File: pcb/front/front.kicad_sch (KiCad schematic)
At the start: 187 parts

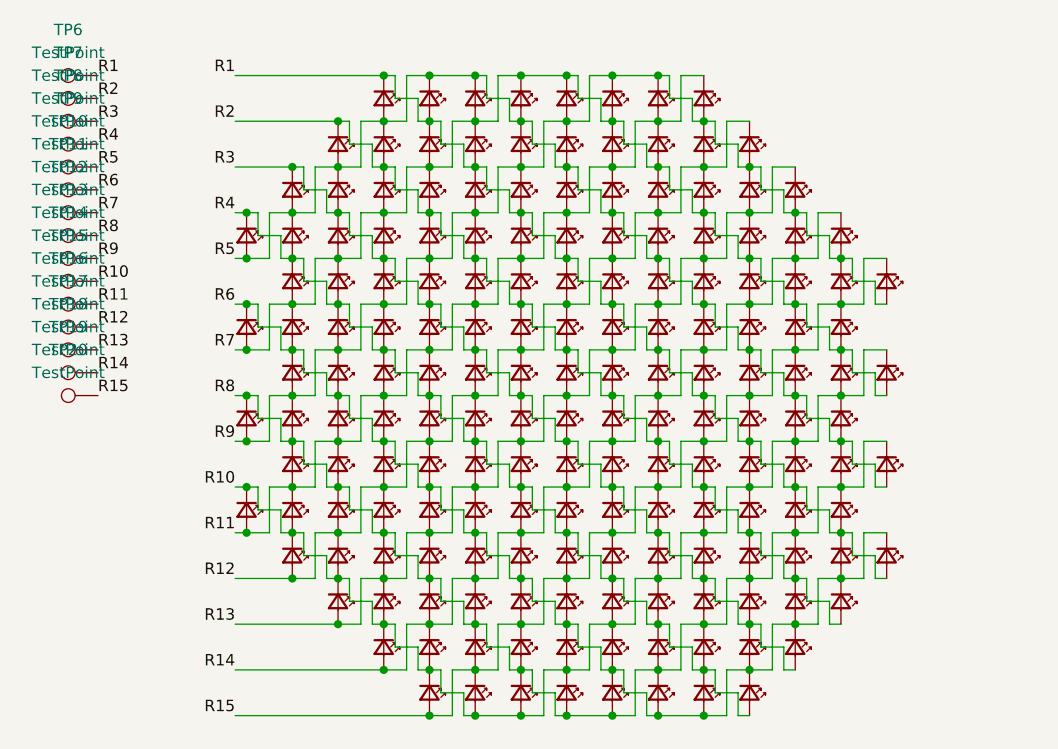
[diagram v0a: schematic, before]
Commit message: Format schematics
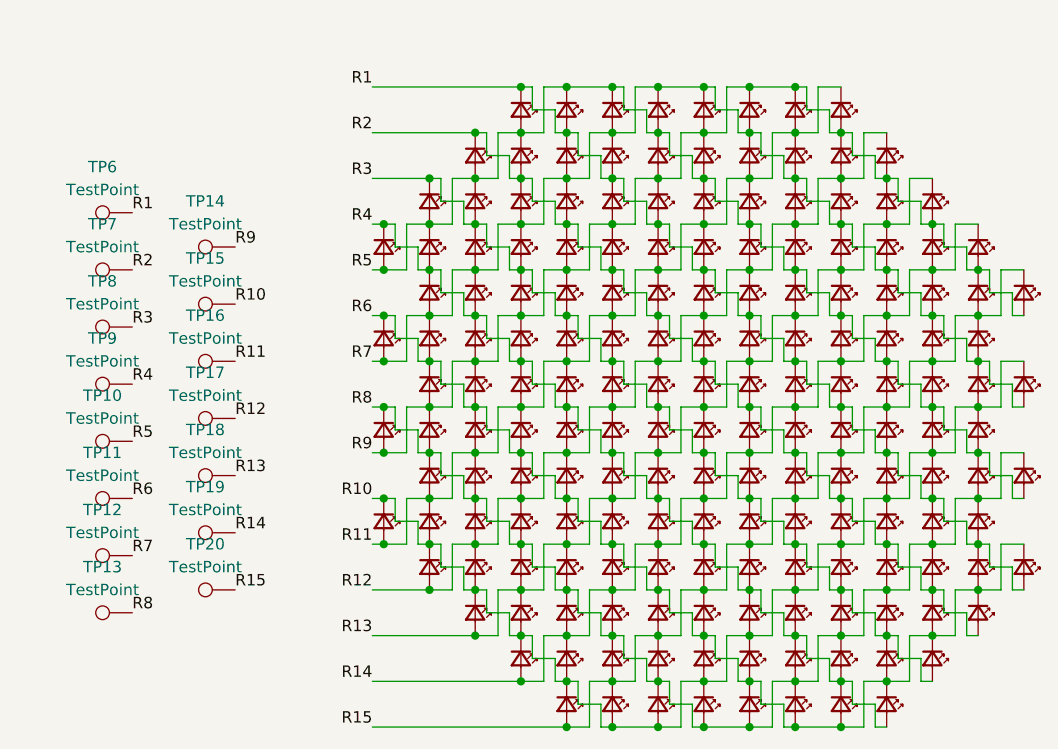
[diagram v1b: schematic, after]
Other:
- moved on the sheet: TP10, TP11, TP12, TP13, TP14, TP15, TP16, TP17, TP18, TP19, TP20, TP6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
